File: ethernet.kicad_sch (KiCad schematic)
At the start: 6 parts, among them IC1 PD69104B1ILQ-TR, J24 0826-1X1T-GH-F, U17 KSZ9897RTXC, Y2 25 MHz

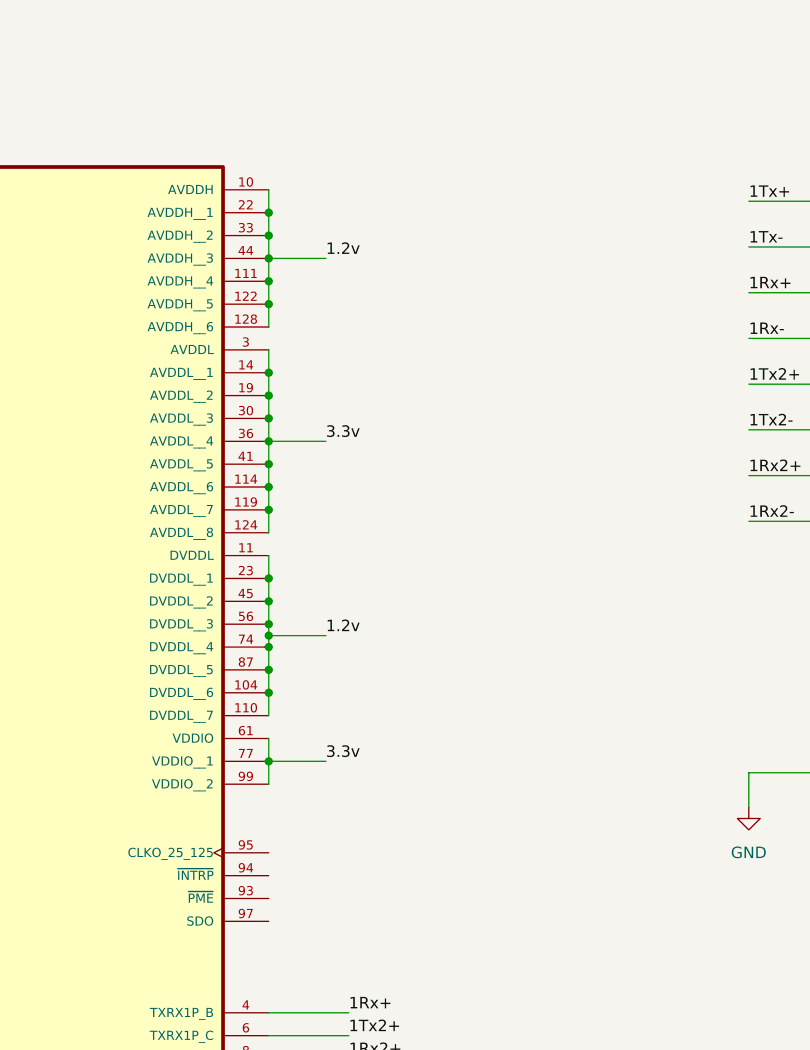
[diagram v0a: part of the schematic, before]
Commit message: stuff
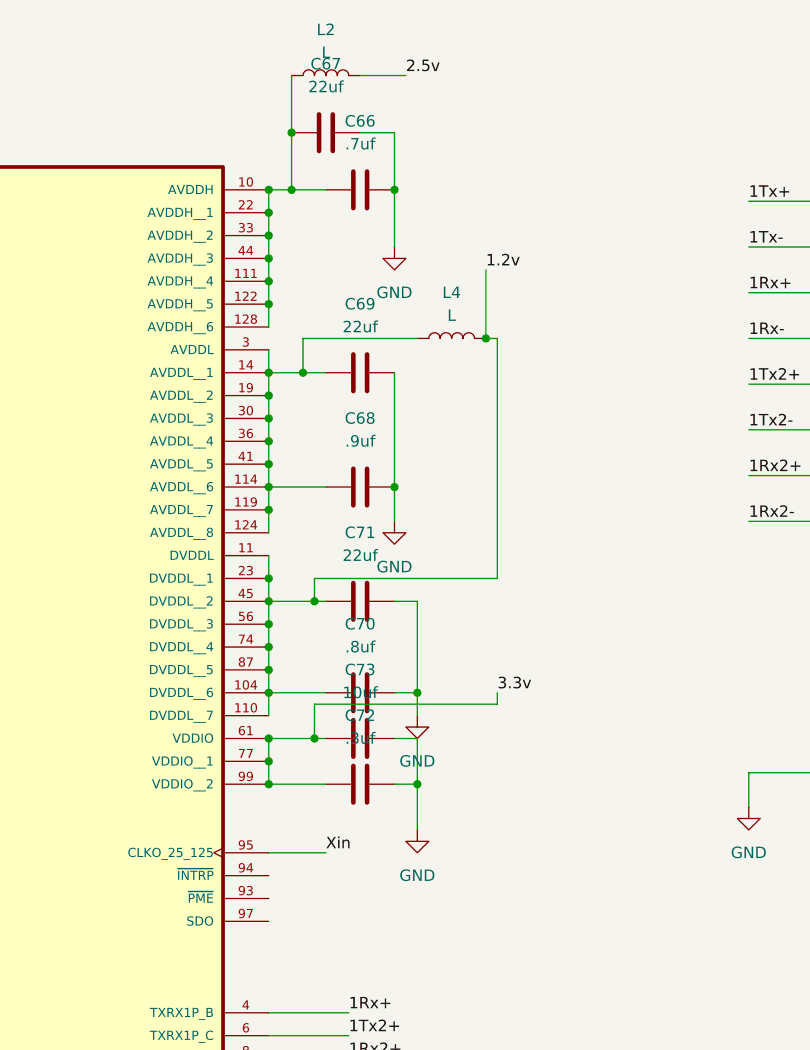
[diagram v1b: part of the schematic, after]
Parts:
- added C66: .7uf, symbol Device:C
- added C67, C69, C71: 22uf, symbol Device:C
- added C68: .9uf, symbol Device:C
- added C70: .8uf, symbol Device:C
- added C72: .3uf, symbol Device:C
- added C73: 10uf, symbol Device:C
- added L2, L4: L, symbol Device:L
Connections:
- net 1.2v: now also C70.1, C71.1, L4.2; no longer U17.10 (AVDDH), U17.111 (AVDDH__4), U17.122 (AVDDH__5), U17.128 (AVDDH__6), U17.22 (AVDDH__1), U17.33 (AVDDH__2), U17.44 (AVDDH__3)
- net 3.3v: now also C72.1, C73.1; no longer U17.114 (AVDDL__6), U17.119 (AVDDL__7), U17.124 (AVDDL__8), U17.14 (AVDDL__1), U17.19 (AVDDL__2), U17.3 (AVDDL), U17.30 (AVDDL__3), U17.36 (AVDDL__4), U17.41 (AVDDL__5)
- net GND: now also C66.2, C67.2, C68.2, C69.2, C70.2, C71.2, C72.2, C73.2
- net Xin: now also U17.95 (CLKO_25_125)
- new net: C68.1, C69.1, L4.1, U17.114 (AVDDL__6), U17.119 (AVDDL__7), U17.124 (AVDDL__8), U17.14 (AVDDL__1), U17.19 (AVDDL__2), U17.3 (AVDDL), U17.30 (AVDDL__3), U17.36 (AVDDL__4), U17.41 (AVDDL__5)
- new net: C66.1, C67.1, L2.1, U17.10 (AVDDH), U17.111 (AVDDH__4), U17.122 (AVDDH__5), U17.128 (AVDDH__6), U17.22 (AVDDH__1), U17.33 (AVDDH__2), U17.44 (AVDDH__3)
- new net 2.5v: L2.2
